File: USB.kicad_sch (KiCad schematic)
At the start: 3 parts, among them J10 USB_OTG, J11 USB_WIFI_FLASH, U9 CP2102N-Axx-xQFN28

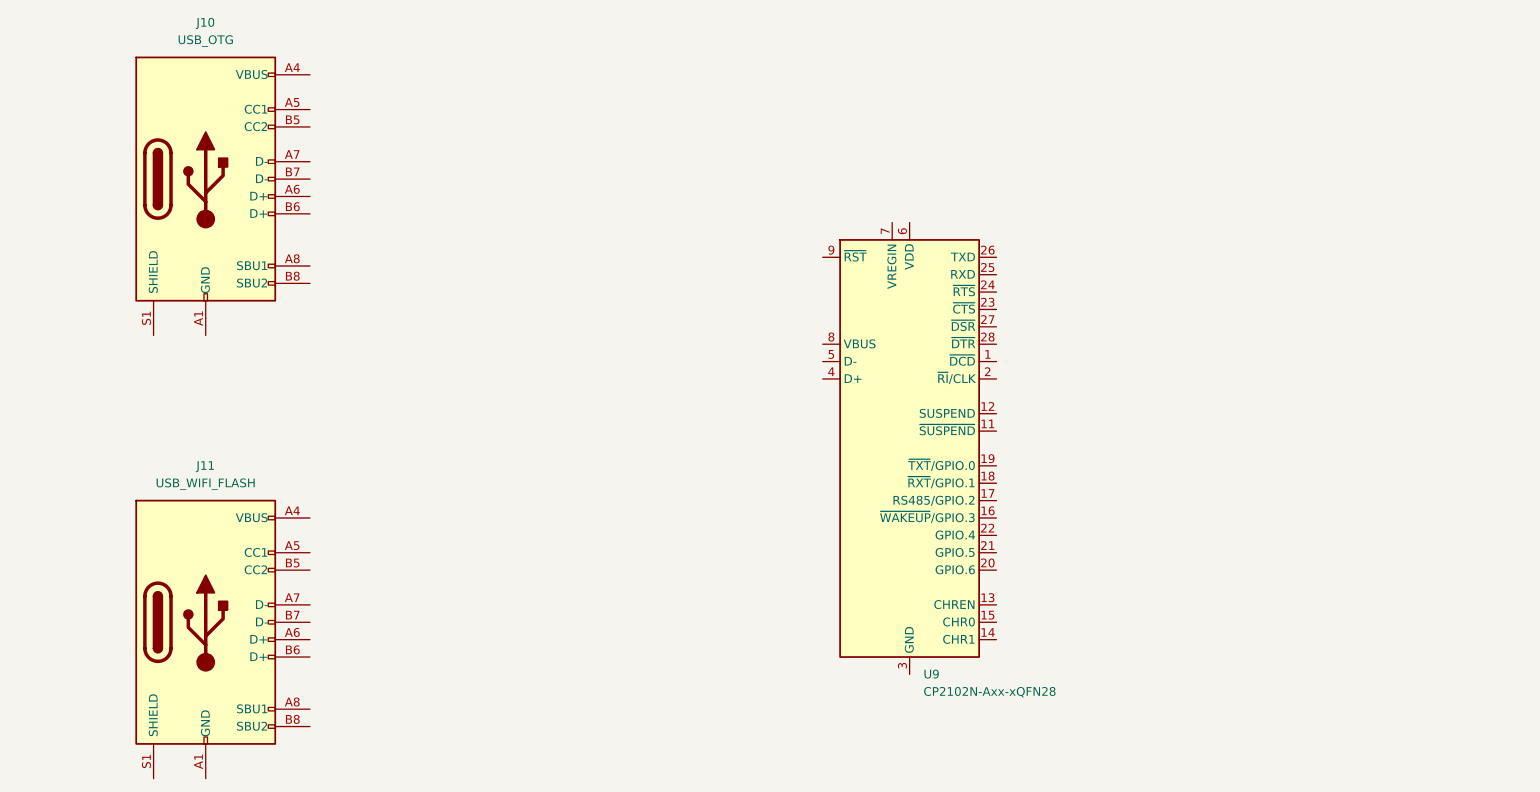
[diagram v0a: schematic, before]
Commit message: Finish USB, LoRa Layout
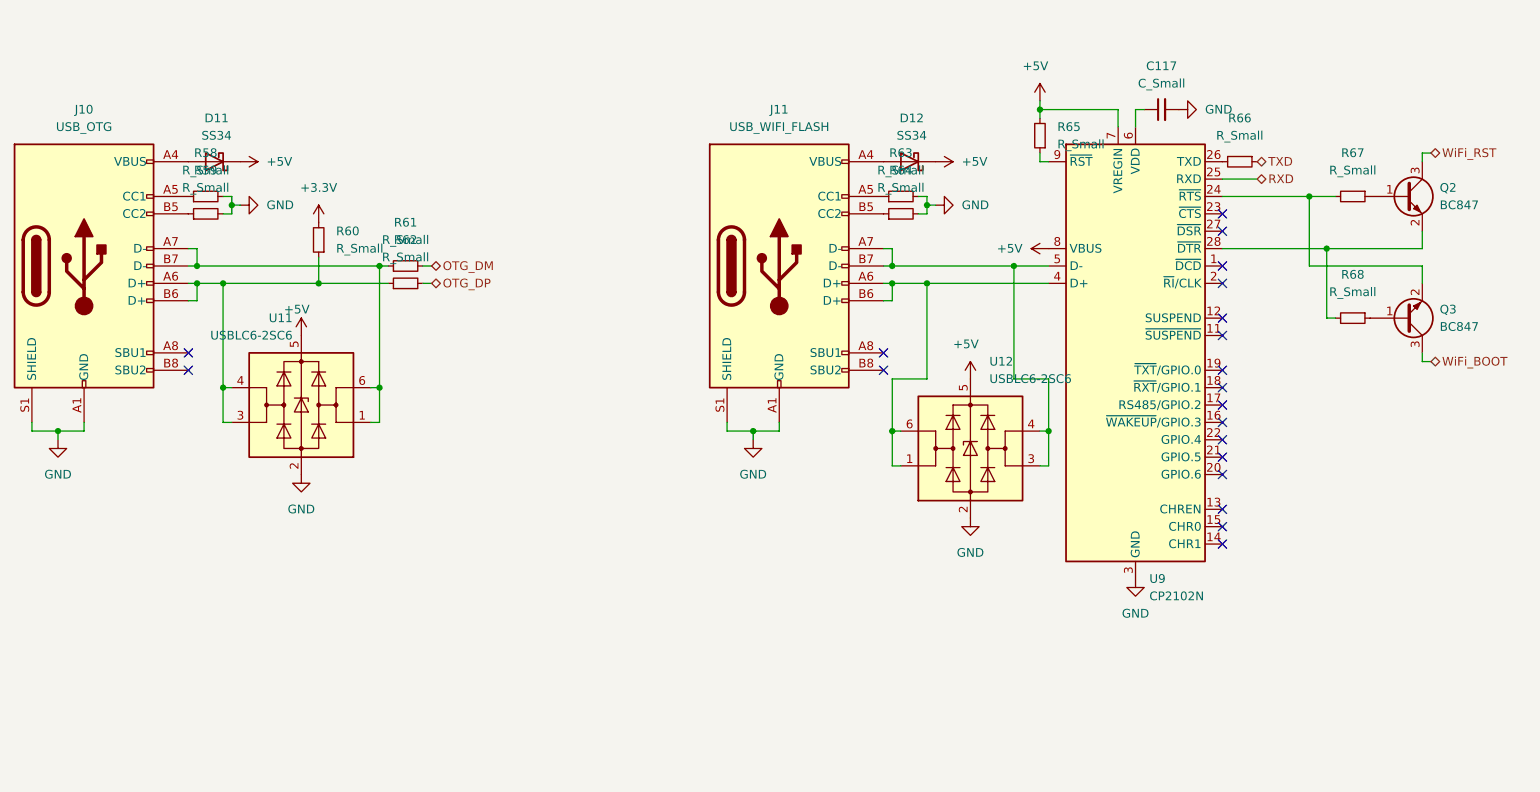
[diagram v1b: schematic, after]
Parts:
- added C117: C_Small, Capacitor_SMD:C_0603_1608Metric, symbol Device:C_Small
- added D11, D12: SS34, Diode_SMD:D_SMA, symbol Diode:CDBA340-HF
- added Q2, Q3: BC847, Package_TO_SOT_SMD:SOT-23, symbol Transistor_BJT:BC847
- added R58, R59, R60, R61, R62, R63, R64, R65, R66, R67, R68: R_Small, Resistor_SMD:R_0603_1608Metric, symbol Device:R_Small
- added U11, U12: USBLC6-2SC6, Package_TO_SOT_SMD:SOT-23-6, symbol Power_Protection:USBLC6-2SC6
- U9: value CP2102N-Axx-xQFN28 -> CP2102N
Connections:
- net GND: now reaches J11.A1 (GND), J11.A12 (GND), J11.B1 (GND), J11.B12 (GND)
- net GND: now also J10.A1 (GND), J10.A12 (GND), J10.B1 (GND), J10.B12 (GND), J10.S1 (SHIELD), J11.S1 (SHIELD), U9.29 (GND), U9.3 (GND), C117.2, R58.2, R59.2, R63.2, R64.2, U11.2 (GND), U12.2 (GND)
- net at J11.A4 (VBUS), J11.A9 (VBUS), J11.B4 (VBUS)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: now also D12.2 (A)
- net at J11.A5 (CC1): now also R63.1
- net at J11.A6 (D+): now also J11.B6 (D+), U9.4 (D+), U12.1 (I/O1), U12.6 (I/O1)
- net at J11.A7 (D-): now also J11.B7 (D-), U9.5 (D-), U12.3 (I/O2), U12.4 (I/O2)
- net at J11.B5 (CC2): now also R64.1
- net at U9.24 (~{RTS}): now also Q3.2 (E), R67.2
- net RXD: now reaches U9.25 (RXD)
- net at U9.26 (TXD): now also R66.2
- net at U9.28 (~{DTR}): now also Q2.2 (E), R68.2
- net at U9.6 (VDD): now also C117.1
- net +5V: now reaches U9.7 (VREGIN)
- net +5V: now also U9.8 (VBUS), D11.1 (K), D12.1 (K), R65.2, U11.5 (VBUS), U12.5 (VBUS)
- net at U9.9 (~{RST}): now also R65.1
- net at J10.A4 (VBUS), J10.A9 (VBUS), J10.B4 (VBUS)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: now also D11.2 (A)
- net at J10.A5 (CC1): now also R58.1
- net at J10.A6 (D+): now also J10.B6 (D+), R60.1, R62.1, U11.3 (I/O2), U11.4 (I/O2)
- net at J10.A7 (D-): now also J10.B7 (D-), R61.1, U11.1 (I/O1), U11.6 (I/O1)
- net at J10.B5 (CC2): now also R59.1
- new net: Q2.1 (B), R67.1
- new net: Q3.1 (B), R68.1
- new net +3.3V: R60.2
- new net OTG_DM: R61.2
- new net OTG_DP: R62.2
- new net TXD: R66.1
- new net WiFi_BOOT: Q3.3 (C)
- new net WiFi_RST: Q2.3 (C)
- no-connect marks 0 -> 20
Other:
- moved on the sheet: J10, J11, U9

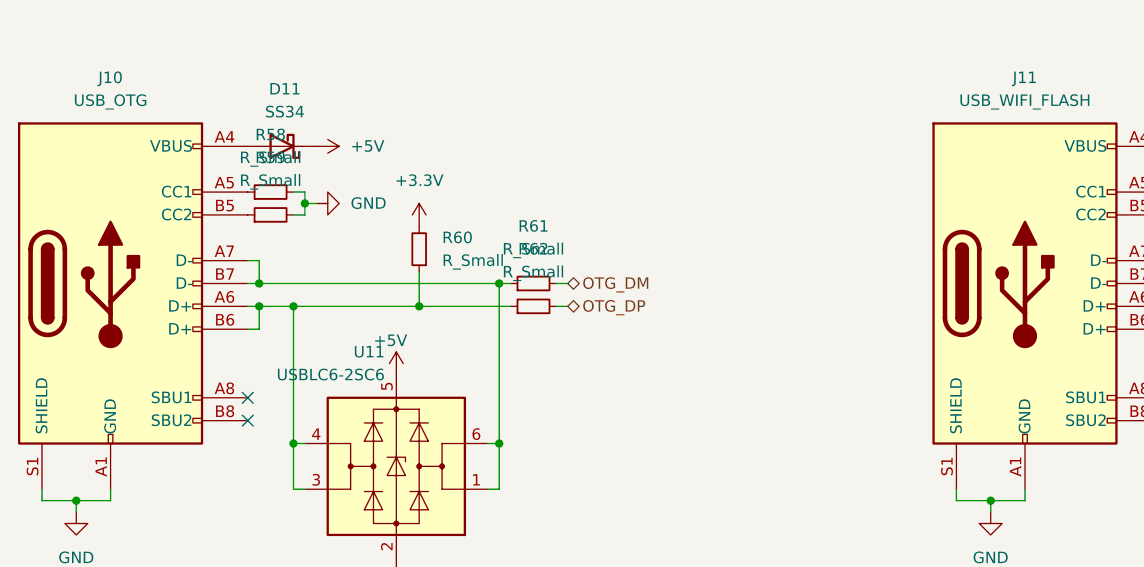
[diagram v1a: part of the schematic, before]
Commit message: Only 1 wire to complete.
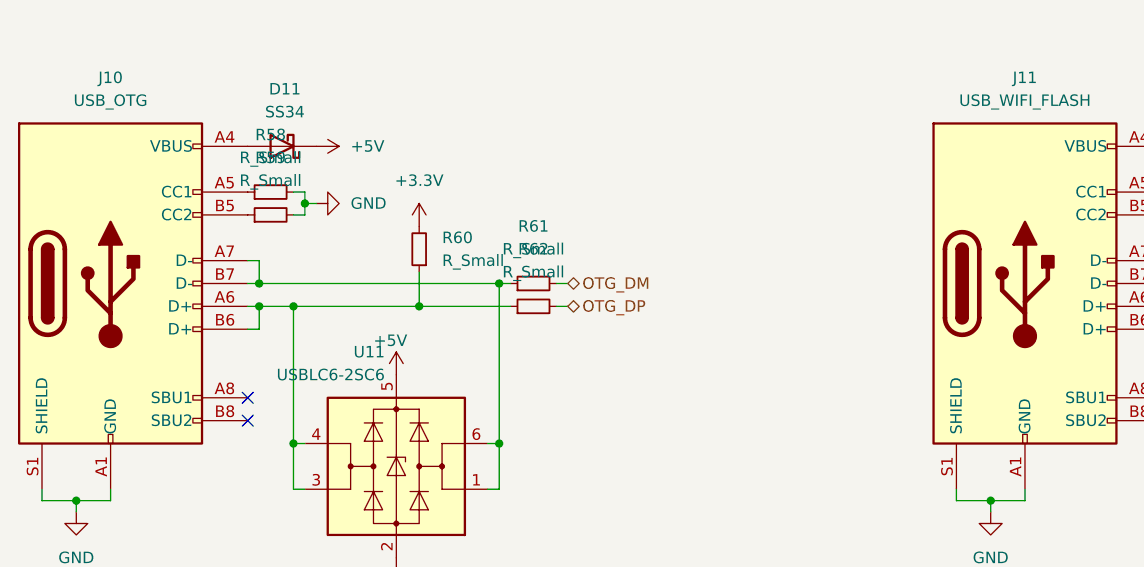
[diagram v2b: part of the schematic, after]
